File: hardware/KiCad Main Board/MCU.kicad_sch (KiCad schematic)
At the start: 67 parts, among them J1 SWD Debug, J2 USB4105, U1 W25Q128JVS, U7 RP2350B-QFN80, Y1 ABM8-272-T3

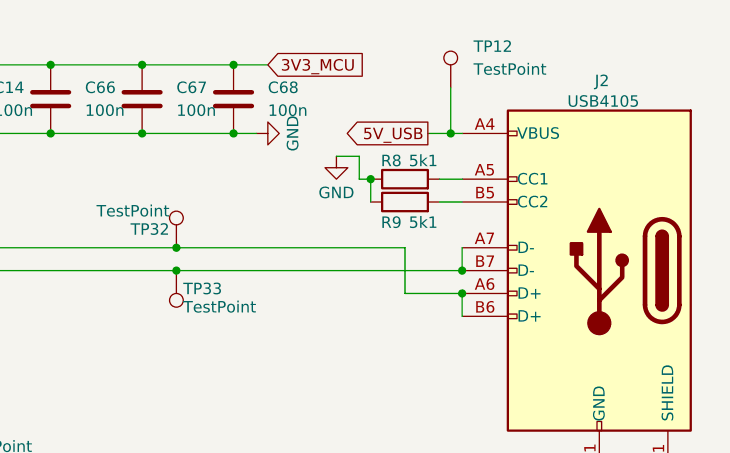
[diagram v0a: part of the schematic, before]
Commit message: did all the things
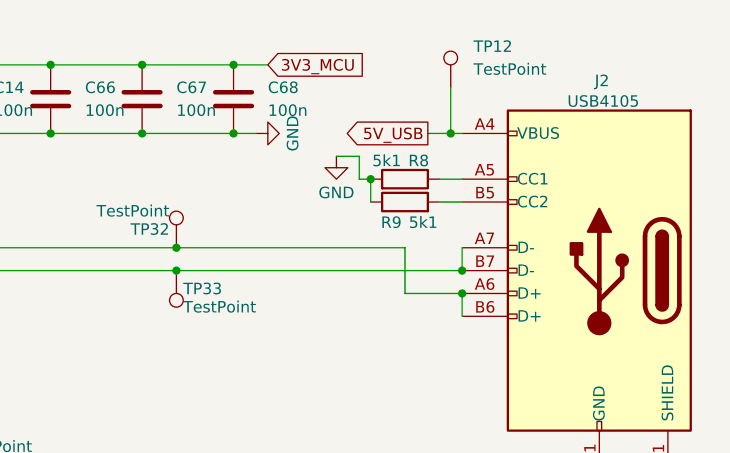
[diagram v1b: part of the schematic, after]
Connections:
- net GND: now also R8.2; no longer R8.1
- net at J2.A5 (CC1): now also R8.1; no longer R8.2
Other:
- moved on the sheet: R8
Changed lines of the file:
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@@
 	(symbol
 		(lib_id "Device:R")
-		(at 241.3 35.56 90)
+		(at 241.3 35.56 270)
+		(mirror x)
 		(unit 1)
 		(exclude_from_sim no)
@@
 		(dnp no)
 		(property "Reference" "R8"
-			(at 239.776 33.528 90)
+			(at 242.824 33.528 90)
 			(effects
 				(font
@@
 		)
 		(property "Value" "5k1"
-			(at 243.332 33.528 90)
+			(at 239.268 33.528 90)
 			(effects
 				(font
